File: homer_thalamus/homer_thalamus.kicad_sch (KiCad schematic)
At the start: 21 parts, among them J1 GPIO, J2 Conn_01x02_Pin, J3 Right_Motor_Conn, J4 Left_Motor_Conn, J5 Spare_Conn, J7 BAT_OUT, J8 BAT_IN, SW1 SW_PULLDOWN, U1 DRV8874_CARRIER_RIGHT, U2 DRV8874_CARRIER_LEFT, U3 HC-SR04, U4 HiLetGo-GY-521

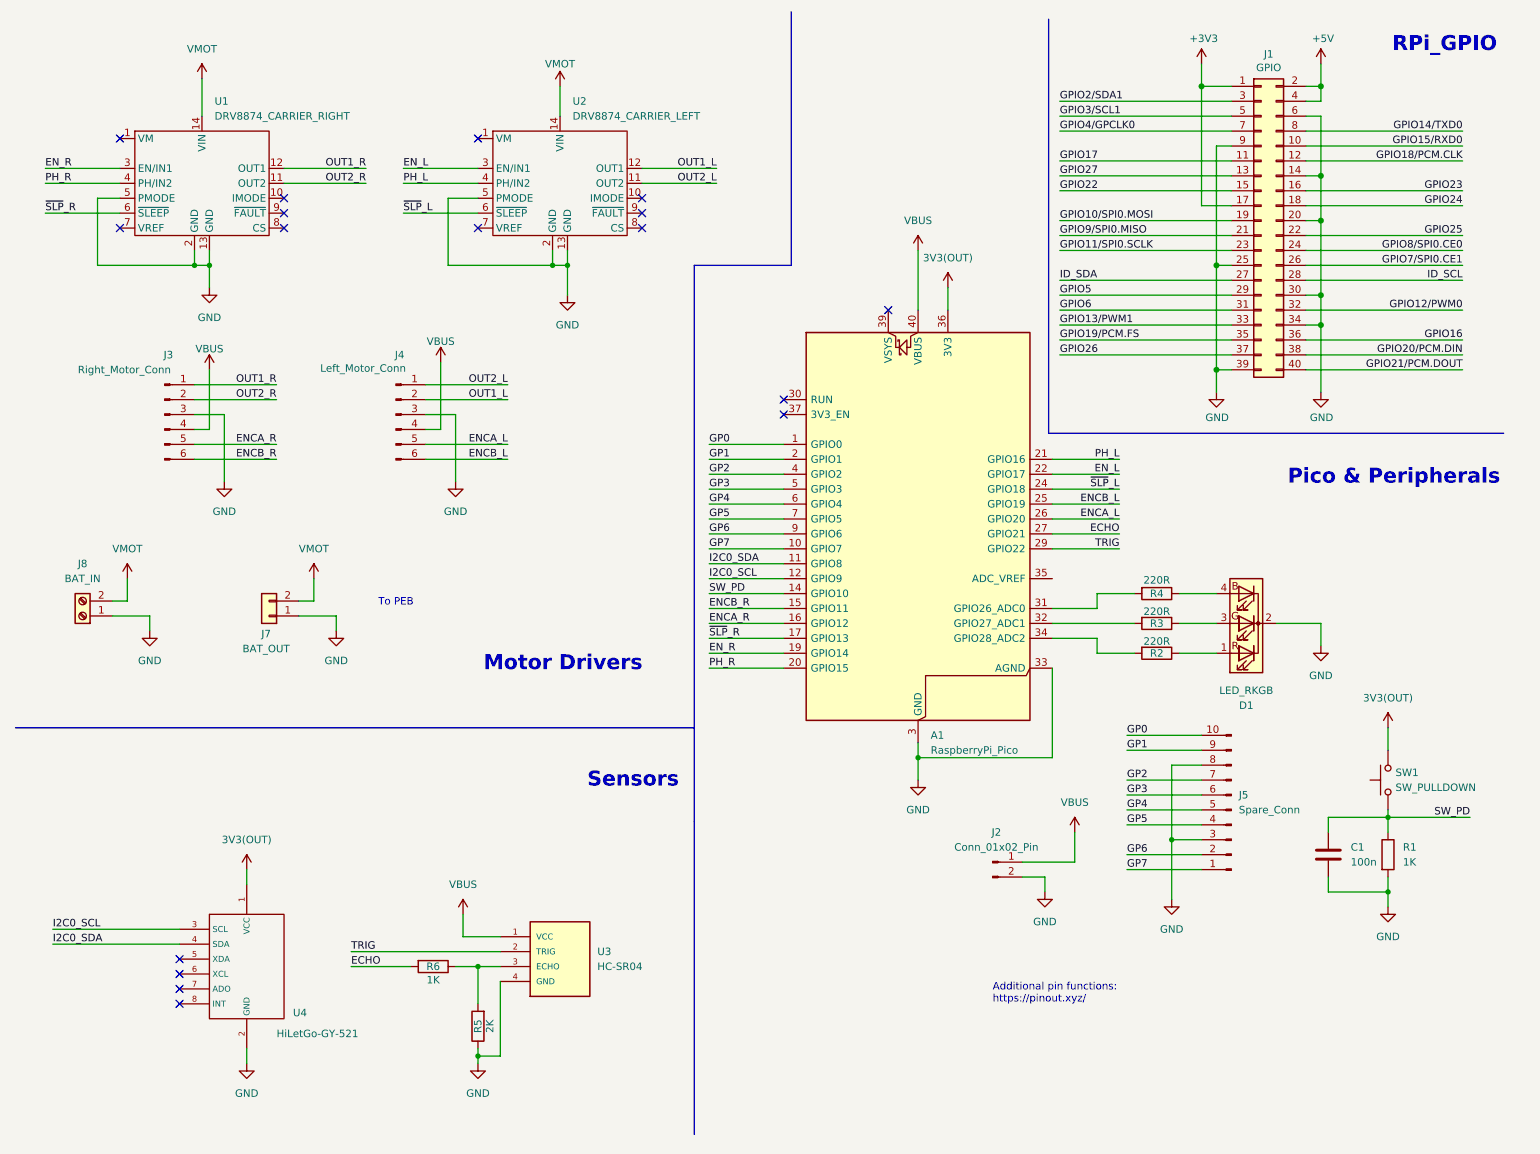
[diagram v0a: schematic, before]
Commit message: reorganize sch
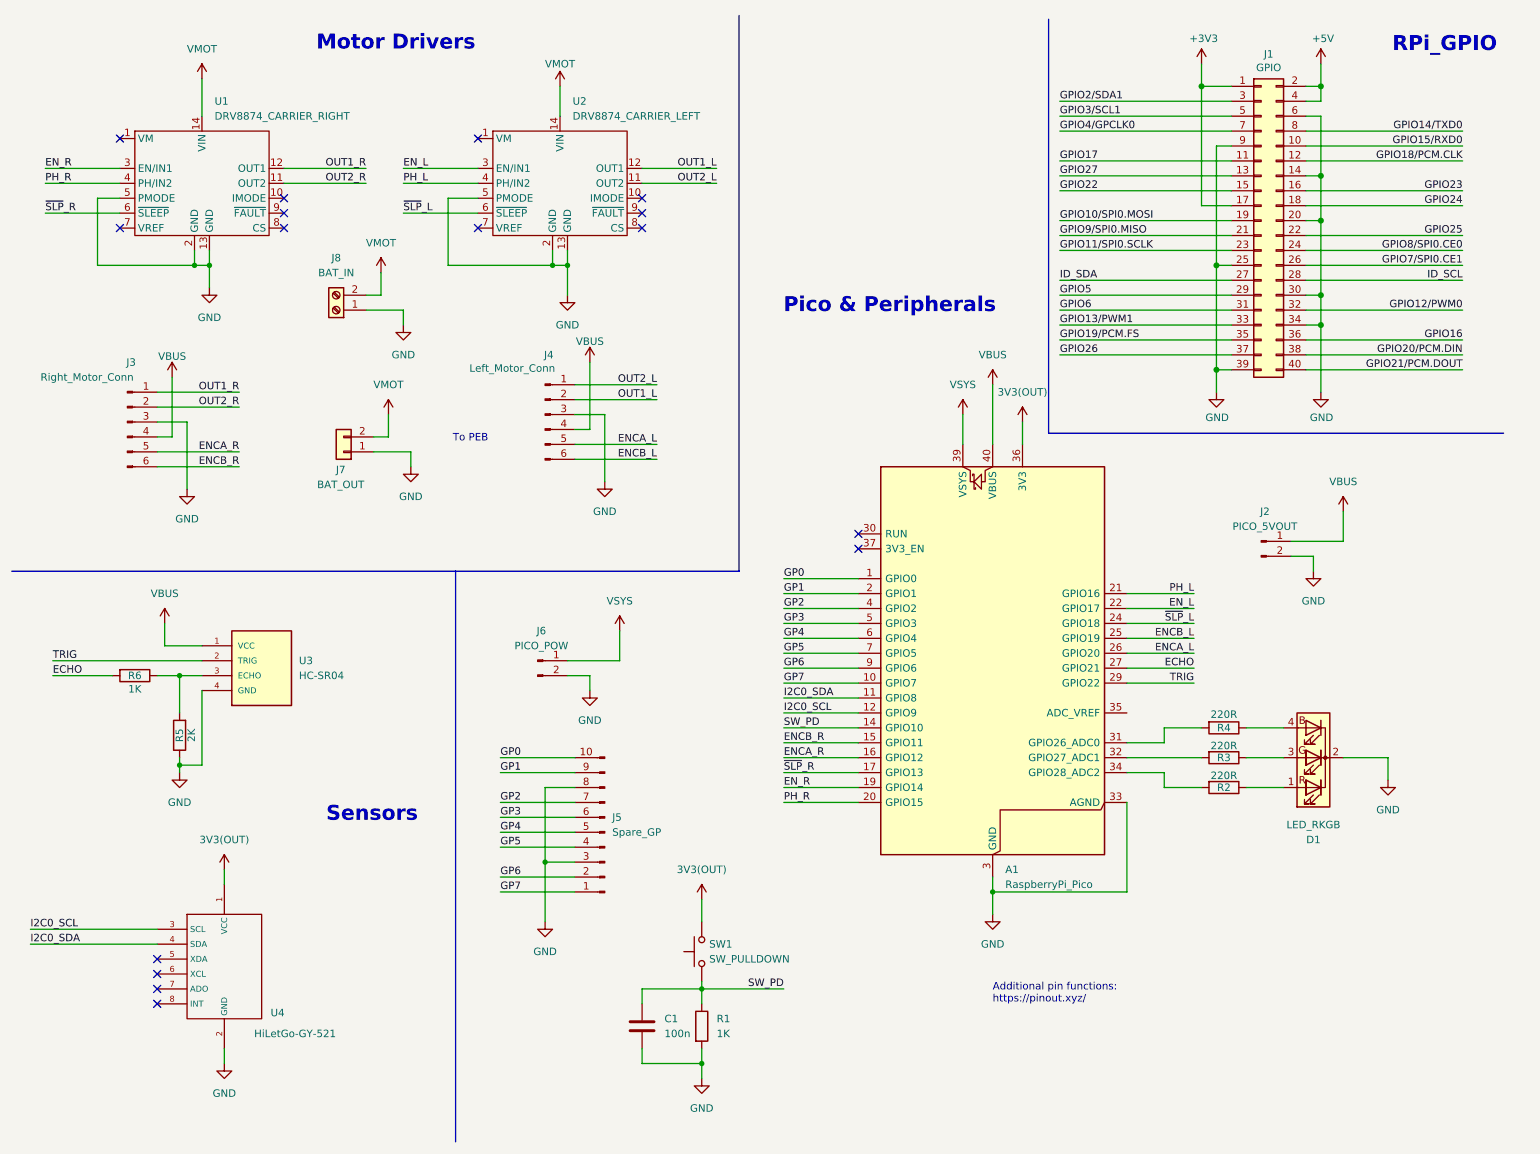
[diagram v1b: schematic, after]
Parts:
- added J6: PICO_POW, symbol Connector:Conn_01x02_Pin
- J2: value Conn_01x02_Pin -> PICO_5VOUT
- J5: value Spare_Conn -> Spare_GP
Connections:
- net GND: now also J6.2 (Pin_2)
- net VSYS: now reaches A1.39 (VSYS)
- net VSYS: now also J6.1 (Pin_1)
- no-connect marks 17 -> 16
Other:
- moved on the sheet: A1, C1, D1, J2, J3, J4, J5, J7, J8, R1, R2, R3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

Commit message: update footprints
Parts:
- J2: footprint (none) -> Connector_PinHeader_2.54mm:PinHeader_1x02_P2.54mm_Vertical
- J6: footprint (none) -> Connector_PinHeader_2.54mm:PinHeader_1x02_P2.54mm_Horizontal
- J8: footprint (none) -> TerminalBlock:TerminalBlock_MaiXu_MX126-5.0-02P_1x02_P5.00mm
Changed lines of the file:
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@@
 			)
 		)
-		(property "Footprint" ""
+		(property "Footprint" "TerminalBlock:TerminalBlock_MaiXu_MX126-5.0-02P_1x02_P5.00mm"
 			(at 67.31 62.23 0)
 			(effects
@@
 			)
 		)
-		(property "Footprint" ""
+		(property "Footprint" "Connector_PinHeader_2.54mm:PinHeader_1x02_P2.54mm_Horizontal"
 			(at 101.6 121.92 0)
 			(effects
@@
 			)
 		)
-		(property "Footprint" ""
+		(property "Footprint" "Connector_PinHeader_2.54mm:PinHeader_1x02_P2.54mm_Vertical"
 			(at 224.79 101.6 0)
 			(effects

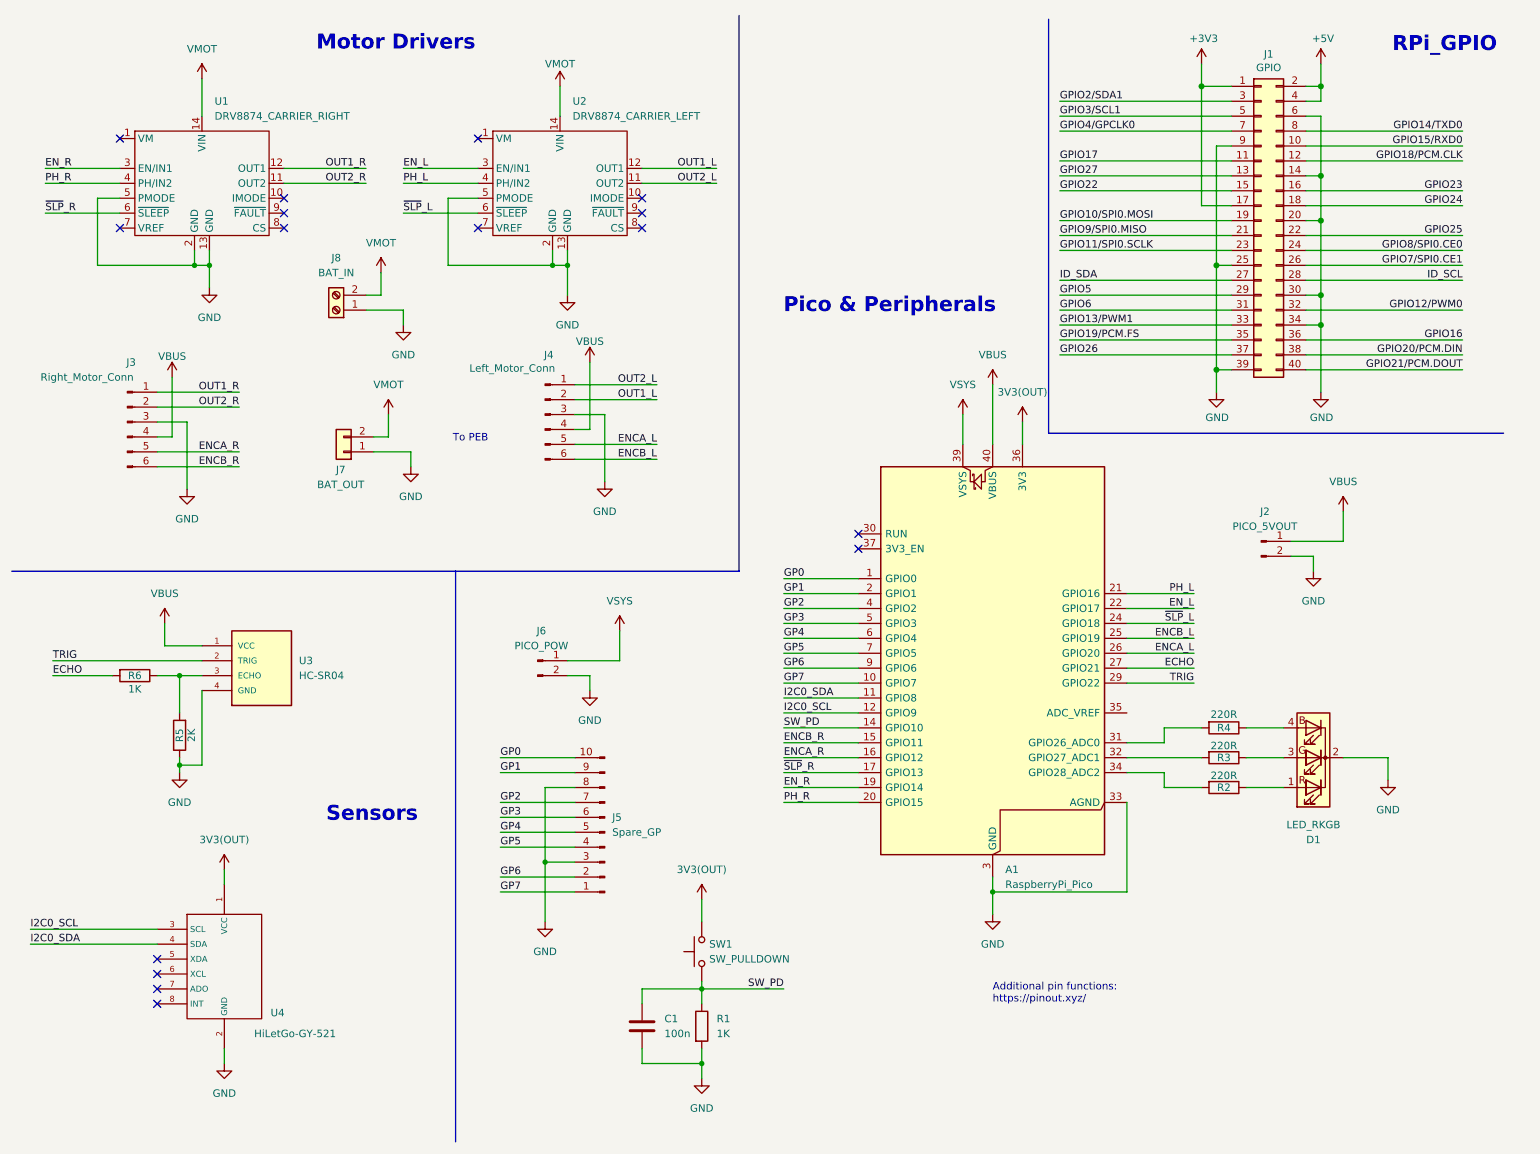
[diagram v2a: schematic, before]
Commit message: reorganize sch
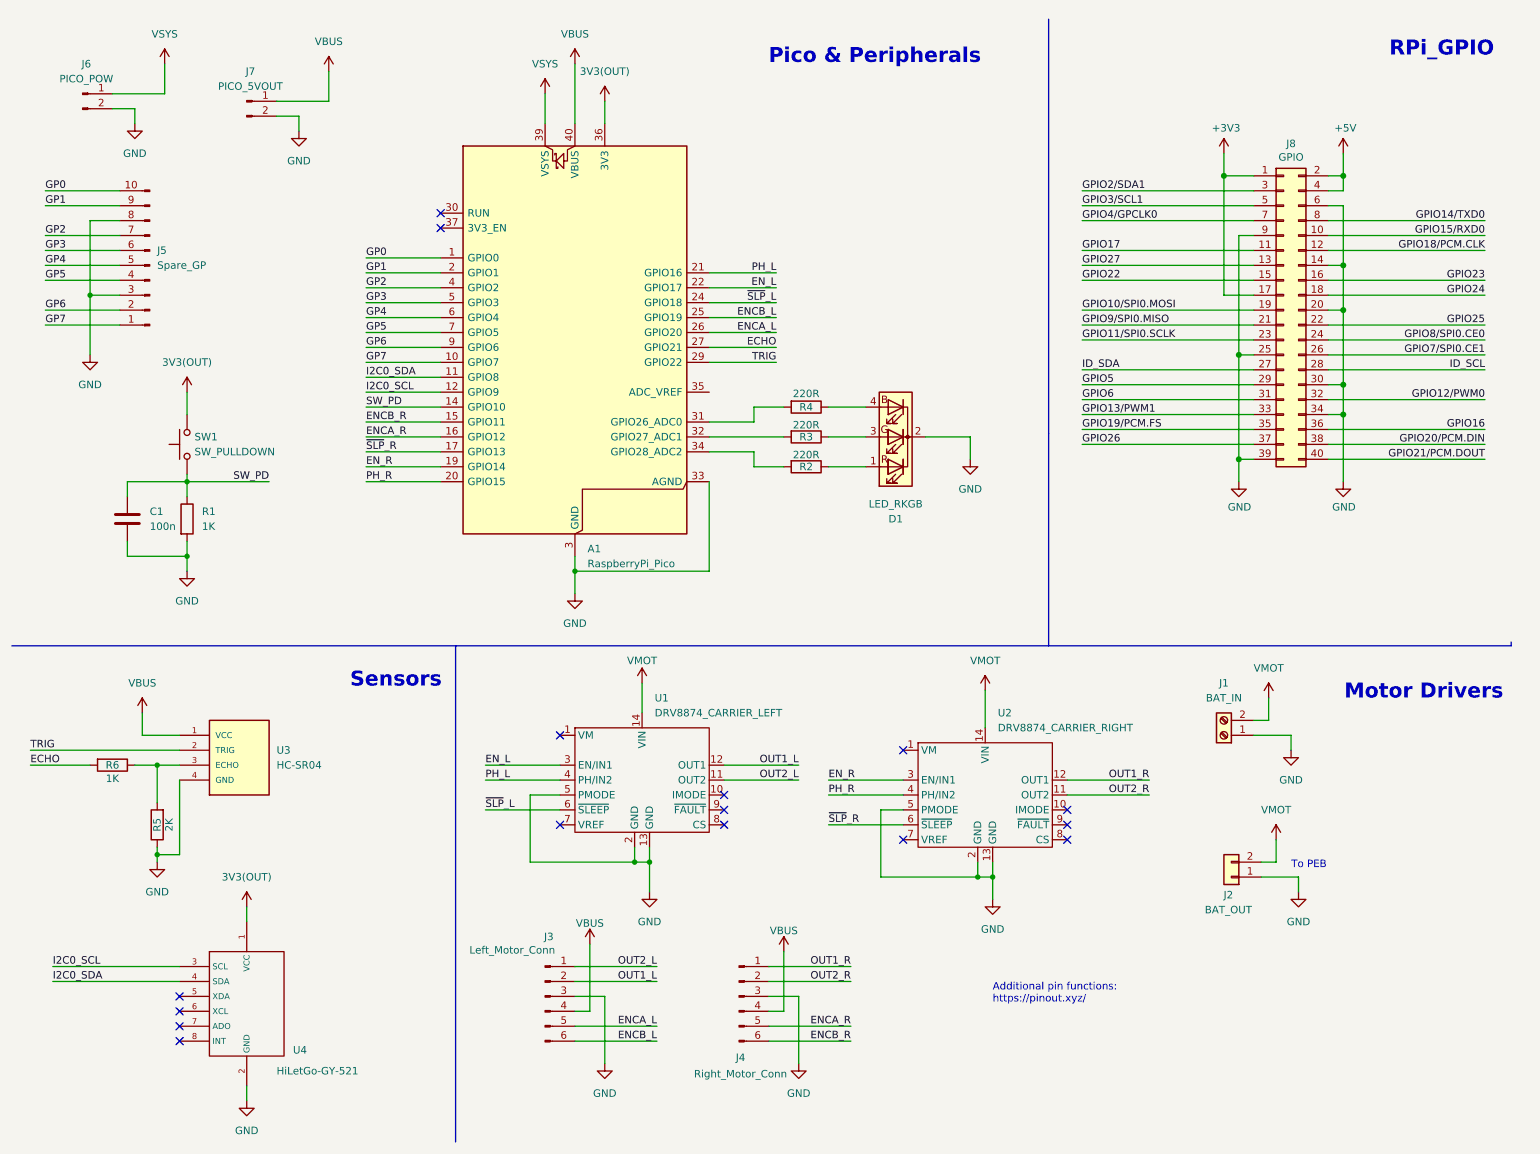
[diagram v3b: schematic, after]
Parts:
- renumbered J8 to J1, J7 to J2, J4 to J3, J3 to J4, J2 to J7, J1 to J8, U2 to U1, U1 to U2
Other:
- moved on the sheet: A1, C1, D1, J1, J2, J3, J4, J5, J6, J7, J8, R1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
